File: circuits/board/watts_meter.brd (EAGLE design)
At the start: 100.3 x 70 mm, 41 parts

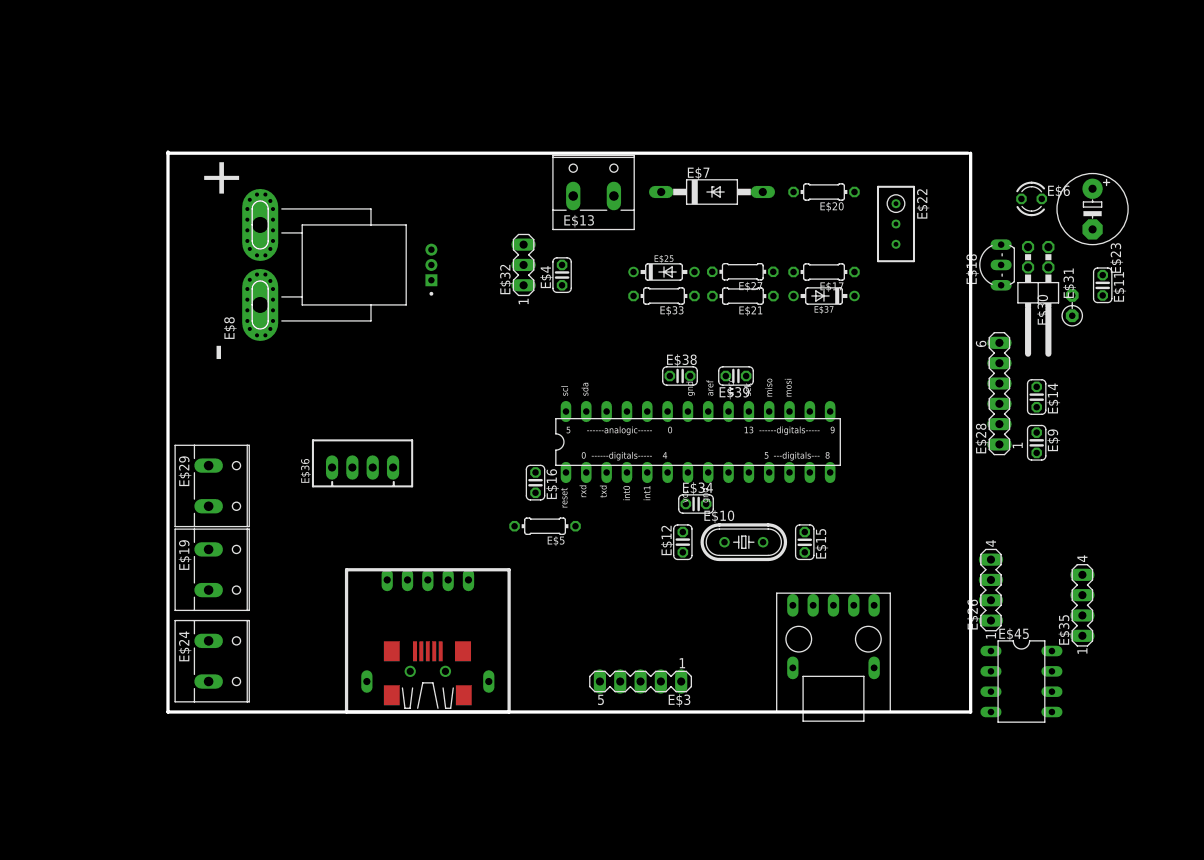
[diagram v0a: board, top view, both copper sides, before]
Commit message: .
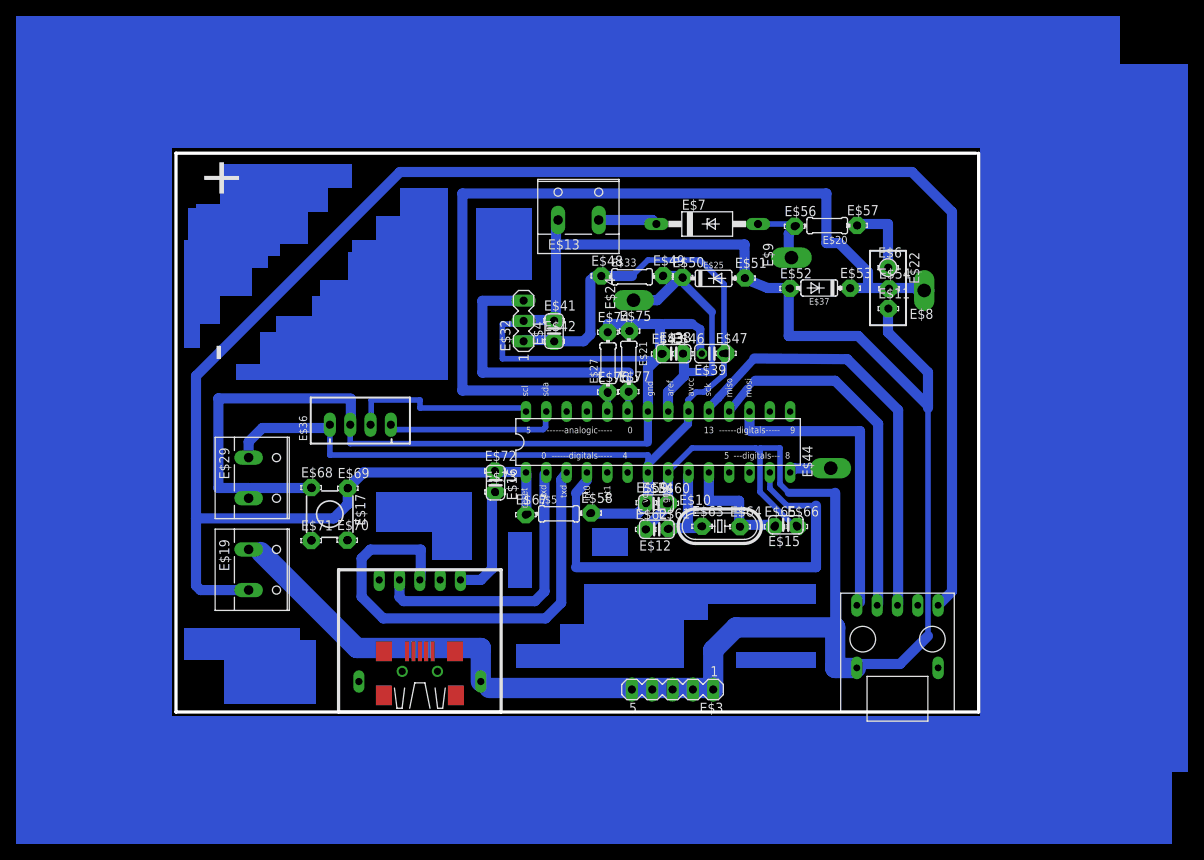
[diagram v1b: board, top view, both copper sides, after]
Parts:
- removed E$14: (no value), rcl:C025-024X044
- removed E$18: (no value), transistor-fet:TO92-
- removed E$23: (no value), ref-packages-longpad:E5-8,5
- removed E$26, E$35: (no value), con-lstb:MA04-1
- removed E$28: (no value), con-lstb:MA06-1
- removed E$30: (no value), discrete:RS-2,5
- removed E$31: (no value), pinhead:2X02/90
- removed E$45: (no value), 74xx-us:DIL08
- added E$41, E$42, E$43, E$46, E$47, E$48, E$49, E$50, E$51, E$52, E$53, E$54, E$56, E$57, E$58, E$59, E$60, E$61, E$62, E$63, E$64, E$65, E$66, E$67, E$68, E$69, E$70, E$71, E$72, E$73, E$74, E$75, E$76, E$77: (no value), solpad:LSP10
- added E$44: tx_to_multiplx, testpad:P1-17Y
- E$11: device rcl:C025-024X044 -> solpad:LSP10
- E$17: value 2.2k -> (none); device eagle-ltspice:0204/7 -> switch:TL1105
- E$24: value 5V -> 123; device con-wago-508:W237-132 -> testpad:P1-17Y
- E$3: value (none) -> ground-group
- E$6: device led:LED3MM -> solpad:LSP10
- E$8: value ACS758LCB 50U -> 123; device ACS758LCB-100B-PFF-T:XDCR_ACS770KCB-150U-PFF-T -> testpad:P1-17Y
- E$9: value (none) -> 123; device rcl:C025-024X044 -> testpad:P1-17Y
- moved E$8 72.4 mm to (94.5, 52.7), turned to 180 degrees
- moved E$24 69.2 mm to (58.2, 51.5), turned to 90 degrees
- moved E$17 68.8 mm to (20.2, 24.7)
- moved E$9 38.4 mm to (77.9, 56.8), turned to 90 degrees
- moved E$11 26.9 mm to (90.0, 50.4), turned to 0 degrees
- moved E$27 20.4 mm to (55.0, 43.6), turned to 90 degrees
- moved E$6 19.9 mm to (90.0, 55.5)
- moved E$21 16.4 mm to (57.6, 43.8), turned to 270 degrees
- moved E$22 8.06 mm to (90.0, 53.0)
- moved PROGRAM 8.00 mm to (91.2, 6.99)
- moved E$4 7.07 mm to (48.3, 47.6)
- moved E$32 7.00 mm to (44.5, 48.9)
- moved E$25 6.25 mm to (68.2, 54.2)
- moved E$36 5.36 mm to (24.0, 35.9)
- moved E$29 5.10 mm to (10.7, 29.3)
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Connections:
- removed net S$22: E$13.1, E$17.2, E$21.1, E$22.3, E$25.A, E$27.2, E$32.2, E$33.1, E$37.A, E$4.2, E$8.2
- removed net S$4: E$1.23, E$21.2, E$8.3
- new net S$18: E$1.22, E$1.8, E$12.2, E$13.1, E$15.1, E$17.4, E$19.1, E$2.P$7, E$21.1, E$22.3, E$25.A, E$27.2, E$29.2, E$3.1, E$3.2, E$3.3, E$3.4, E$3.5, E$32.2, E$34.2, E$36.2, E$37.A, E$38.1, E$39.2, E$4.2, PROGRAM.P$6
- new net S$23: E$1.24, E$22.2, E$27.1, E$37.C, E$8.TP
- new net S$24: E$1.21, E$24.TP, E$25.C, E$33.2, E$38.2
- net 5V: now also E$1.20, E$1.7, E$33.1, E$34.1, E$39.1, E$5.2; no longer E$1.21, E$25.C, E$33.2, E$38.2, E$8.1
- net S$13: no longer E$24.2
- net S$19: now also E$1.14, E$44.TP; no longer E$1.24, E$17.1, E$22.2, E$27.1, E$37.C
- net S$20: now also E$1.13, E$1.4; no longer E$1.22, E$1.8, E$12.2, E$15.1, E$19.1, E$2.P$7, E$24.1, E$29.2, E$3.1, E$3.2, E$3.3, E$3.4, E$3.5, E$34.2, E$36.2, E$38.1, E$39.2, E$5.2, PROGRAM.P$6
- net S$21: now also E$1.23, E$21.2, E$32.3; no longer E$1.20, E$1.7, E$34.1, E$39.1
- net S$7: now also E$17.3
- net S$8: now also E$9.TP
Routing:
- net S$18: track 0.00 -> 437.4 mm
- net S$7: track 0.00 -> 240.2 mm
- net 5V: track 0.00 -> 132.8 mm
- net S$23: track 0.00 -> 115.1 mm
- net S$13: track 0.00 -> 59.9 mm
- net S$20: track 0.00 -> 58.7 mm
- net S$12: track 0.00 -> 53.9 mm
- net S$11: track 0.00 -> 45.4 mm
- net S$10: track 0.00 -> 38.1 mm
- net S$21: track 0.00 -> 37.3 mm
- net S$14: track 0.00 -> 36.0 mm
- net S$24: track 0.00 -> 34.8 mm
- net S$15: track 0.00 -> 23.9 mm
- net S$16: track 0.00 -> 22.1 mm
- net S$3: track 0.00 -> 15.1 mm
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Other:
- board size 100.3 x 70 mm -> 100.3 x 69.8 mm
